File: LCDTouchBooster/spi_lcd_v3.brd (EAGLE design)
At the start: 49.6 x 49.7 mm, 28 parts, among them IC1 REG1117

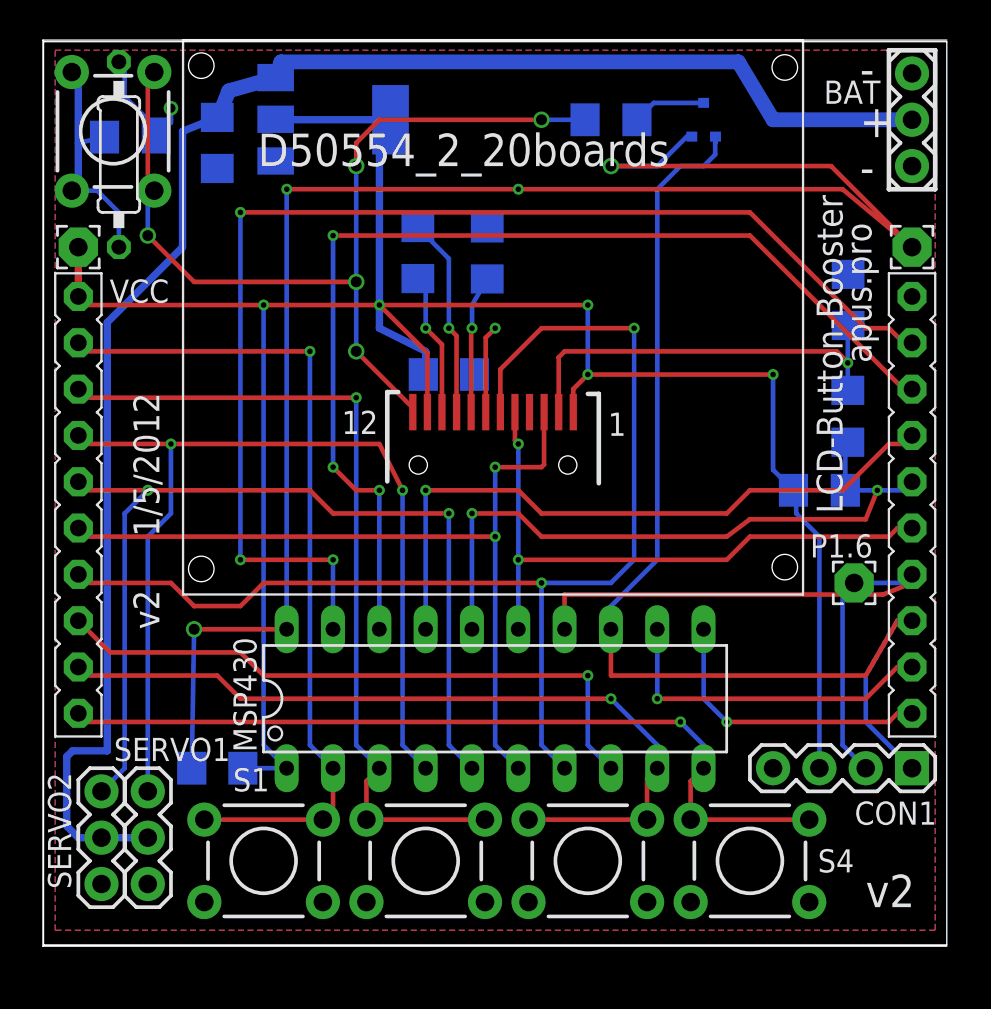
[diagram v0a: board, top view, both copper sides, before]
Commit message: Various changes
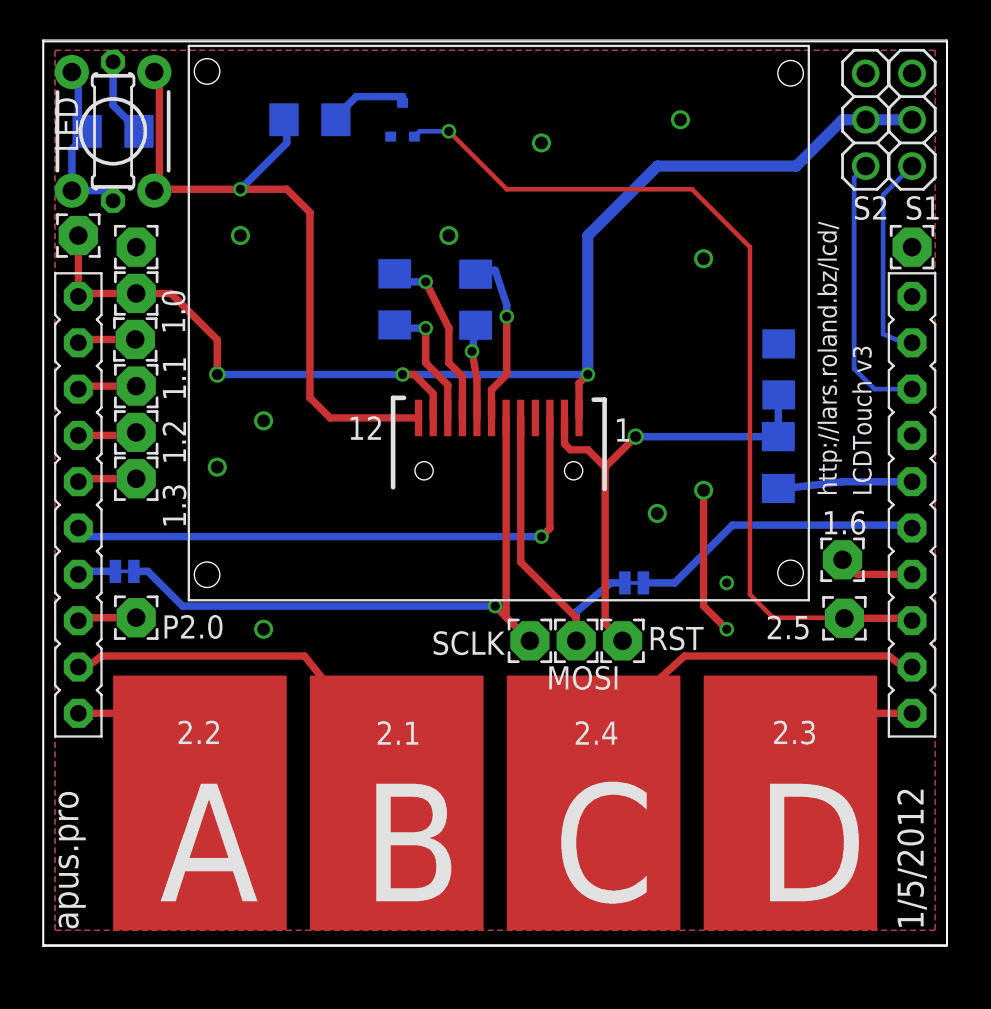
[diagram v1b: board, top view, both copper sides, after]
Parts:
- removed BAT, SERVO1, SERVO2: (no value), SparkFun-Connectors:1X03
- removed C4, C5, C6: (no value), SparkFun:1206
- removed CON1: (no value), SparkFun-Connectors:1X04
- removed IC1: REG1117, burr-brown:SOT223
- removed MSP430: (no value), TI_MSP430_v16:N20
- removed P1.6: (no value), wirepad:2,15/1,0
- removed R2: (no value), resistor:R1206
- removed S3, S4: (no value), SparkFun-Electromechanical:TACTILE-PTH
- added 1.0, 1.1, 1.2, 1.3, 1.6, 2.5, GND3, MOSI, P2.0, RST, SCLK, VCC1: (no value), wirepad:2,15/1,0
- added 2.1, 2.2, 2.3, 2.4: TPTP07R, testpad:TP07R
- added SJ1, SJ2: (no value), SparkFun-Passives:SJ_2S-TRACE
- RLED2: device resistor:0207/10 -> resistor:0207/7
- S1, S2: device SparkFun-Electromechanical:TACTILE-PTH -> adafruit:1X03
- moved S1 54.0 mm to (48.3, 45.7), turned to 270 degrees
- moved S2 47.3 mm to (45.7, 45.7), turned to 270 degrees
- moved LEDSW 16.5 mm to (20.3, 45.7)
- moved RLED1 16.5 mm to (15.2, 45.7)
- moved C3 5.39 mm to (40.9, 32.0)
- moved R1 4.58 mm to (40.9, 26.9)
- moved C2 2.84 mm to (19.9, 35.9)
- moved C1 2.62 mm to (24.3, 35.9)
- moved RLED2 1.31 mm to (4.45, 45.1)
- moved RLED 1.00 mm to (4.45, 45.1), turned to 180 degrees
- moved VCC 0.63 mm to (2.54, 39.4)
- moved U$1 0.45 mm to (25.6, 29.4)
- turned LED to 270 degrees
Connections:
- removed net CSB: LAUNCHPAD.P1.4, MSP430.6, U$1.3
- removed net KBL: LED.3, LED.4, RLED1.2, U$1.12
- removed net N$22 (its old number): LAUNCHPAD.P2.0, MSP430.8
- removed net P1.0: LAUNCHPAD.P1.0, MSP430.2, S1.3, S1.4
- removed net P1.1: LAUNCHPAD.P1.1, MSP430.3, S2.3, S2.4
- removed net P1.2: LAUNCHPAD.P1.2, MSP430.4, SERVO1.1
- removed net P1.3: LAUNCHPAD.P1.3, MSP430.5, SERVO2.1
- removed net VBAT: BAT.2, C5.1, IC1.3, SERVO1.2, SERVO2.2
- removed net VDD: C4.2, C6.2, CON1.3, IC1.2, LAUNCHPAD.VCC, MSP430.1, R2.2, U$1.1, U$1.11, VCC.1
- new net N$16: 2.3.TP, LAUNCHPAD.P2.3
- new net N$17: 1.3.1, LAUNCHPAD.P1.3
- new net N$18: LAUNCHPAD.P2.0, P2.0.1
- new net N$19: 1.1.1, LAUNCHPAD.P1.1
- new net N$23: LAUNCHPAD.P2.7, S2.3
- new net N$24: LED.3, LED.4, RLED.1, RLED2.1
- new net N$25: LED.1, LED.2, RLED1.2, U$1.12
- new net N$9: LAUNCHPAD.P1.4, U$1.3
- new net VCC: LAUNCHPAD.VCC, S1.2, S2.2, U$1.1, U$1.11, VCC.1, VCC1.1
- net GND: now also GND3.1, RLED.2; no longer BAT.3, C4.1, C5.2, C6.1, CON1.4, IC1.1, MSP430.20, RLED.1, S1.2, S2.2, S3.1, S3.2, S4.1, S4.2, SERVO1.3, SERVO2.3
- net N$10: now also LAUNCHPAD.RST, R1.1; no longer LAUNCHPAD.TEST, MSP430.17
- net N$11: now also 1.6.1, LAUNCHPAD.P1.6; no longer LAUNCHPAD.P2.2, MSP430.10, S4.3, S4.4
- net N$12: now also 1.2.1, LAUNCHPAD.P1.2; no longer CON1.2, LAUNCHPAD.P1.6, MSP430.14, P1.6.1
- net N$13: now also 2.1.TP, LAUNCHPAD.P2.1; no longer CON1.1, LAUNCHPAD.P2.5, LEDSW.1, MSP430.13
- net N$14: now also 2.2.TP, LAUNCHPAD.P2.2; no longer LAUNCHPAD.P2.4, MSP430.12
- net N$15: now also 2.4.TP, LAUNCHPAD.P2.4; no longer LAUNCHPAD.P2.3, MSP430.11
- net N$20: now also LAUNCHPAD.P1.7, SJ2.1; no longer LAUNCHPAD.P2.1, MSP430.9, S3.3, S3.4
- net N$21: now also SJ1.2; no longer MSP430.7, U$1.6
- net N$26: now also LAUNCHPAD.P2.6, S1.3; no longer LED.1, LED.2, RLED.2, RLED2.1
- net N$4: now also 2.5.1, LAUNCHPAD.P2.5, LEDSW.1; no longer LAUNCHPAD.P2.6, MSP430.19
- net N$5: now also RST.1
- net N$6: now also 1.0.1, LAUNCHPAD.P1.0; no longer LAUNCHPAD.P2.7, MSP430.18
- net N$7: now also SCLK.1, SJ1.1, U$1.6; no longer LAUNCHPAD.RST, MSP430.16, R1.1, R2.1
- net N$8: now also MOSI.1, SJ2.2; no longer LAUNCHPAD.P1.7, MSP430.15
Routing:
- net VDD: track 127.4 -> 0.00 mm, vias 5 -> 0
- net VBAT: track 90.4 -> 0.00 mm
- net GND: track 108.2 -> 22.2 mm, vias 6 -> 13
- net VCC: track 0.00 -> 68.4 mm, vias 0 -> 3
- net N$21: track 66.3 -> 2.10 mm, vias 2 -> 0
- net N$6: track 59.3 -> 3.20 mm, vias 3 -> 0
- net P1.2: track 54.9 -> 0.00 mm, vias 2 -> 0
- net P1.3: track 53.1 -> 0.00 mm, vias 2 -> 0
- net KBL: track 51.2 -> 0.00 mm, vias 5 -> 0
- net P1.0: track 46.0 -> 0.00 mm, vias 1 -> 0
- net P1.1: track 45.9 -> 0.00 mm, vias 1 -> 0
- net CSB: track 45.7 -> 0.00 mm, vias 2 -> 0
- net N$13: track 61.6 -> 19.3 mm
- net N$11: track 46.2 -> 4.14 mm, vias 1 -> 0
- net N$25: track 0.00 -> 37.2 mm, vias 0 -> 1
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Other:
- board text added: "A"
- board text added: "B"
- board text added: "C"
- board text added: "D"
- board text added: "LCD-Touch"
- board text added: "LCDTouch v3"
- board text removed: "+"
- board text removed: "-"
- board text removed: "D50554_2_20boards"
- board text removed: "LCD-Button-Booster"
- board text removed: "LCD-Button-Boosterpack"
- board text removed: "v2"
